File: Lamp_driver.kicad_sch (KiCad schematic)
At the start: 118 parts, among them J302 T44007, J303 T44007, J304 10146581-060_M, J305 T44007, J306 T44007, Q100 MDT7N65, Q301 MPF3N150, Q303 IXYH55N120, Q304 IXYH55N120, Q305 IXYH55N120, U301 IRS2184

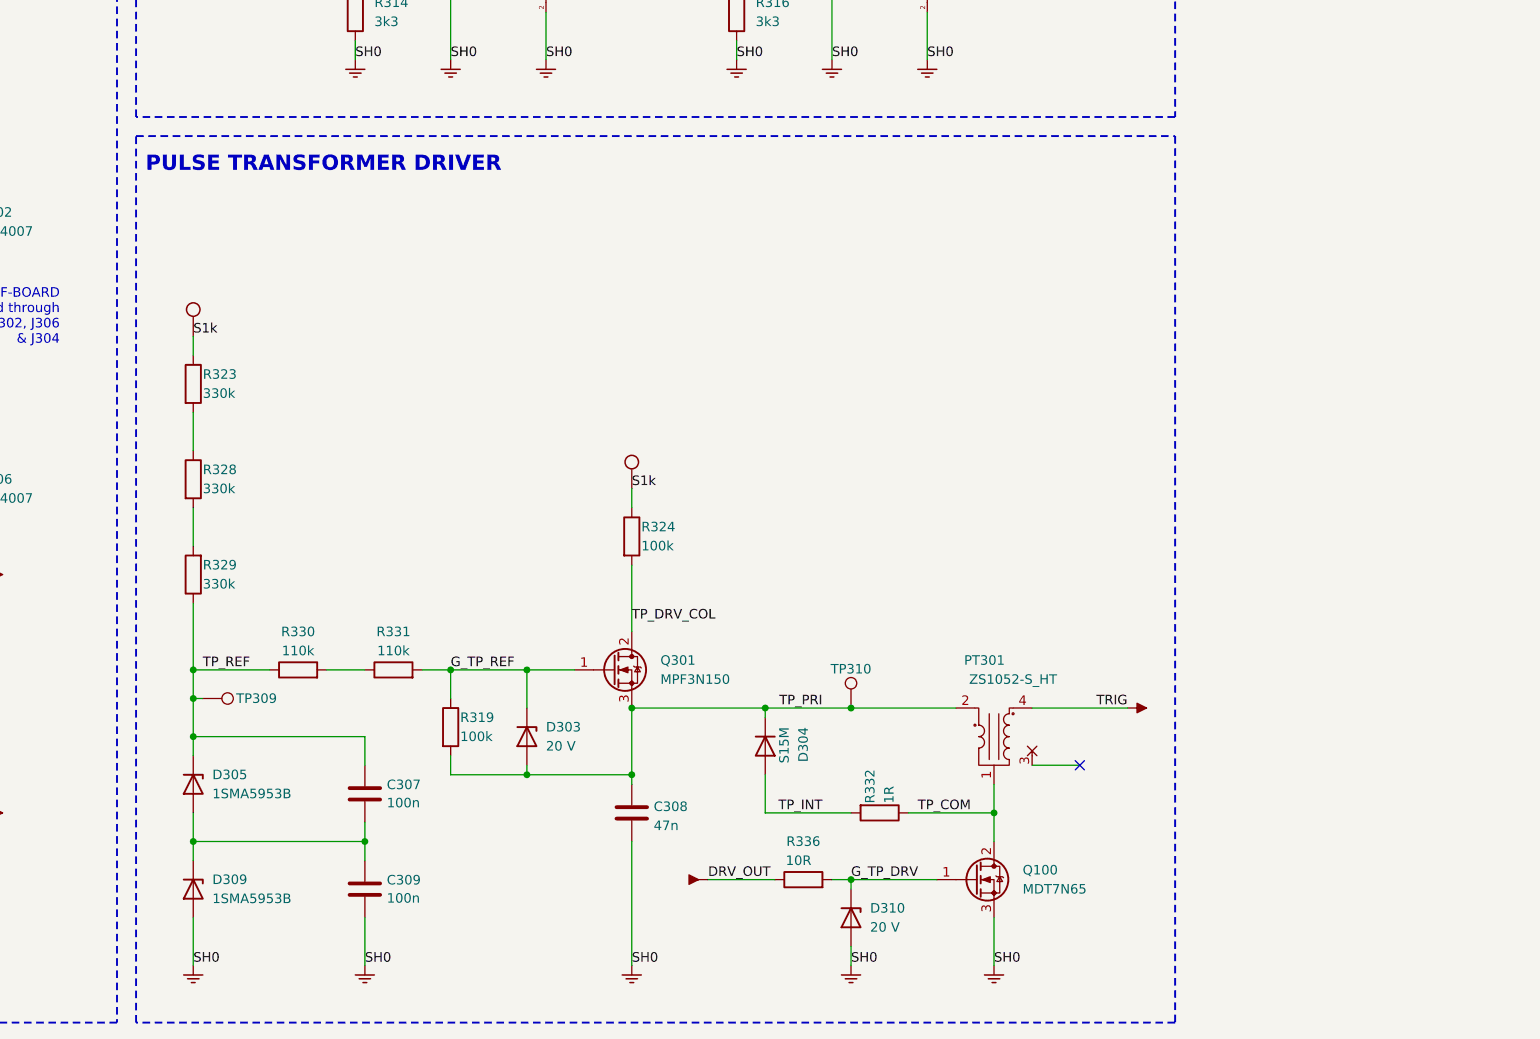
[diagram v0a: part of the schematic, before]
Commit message: Placement updates
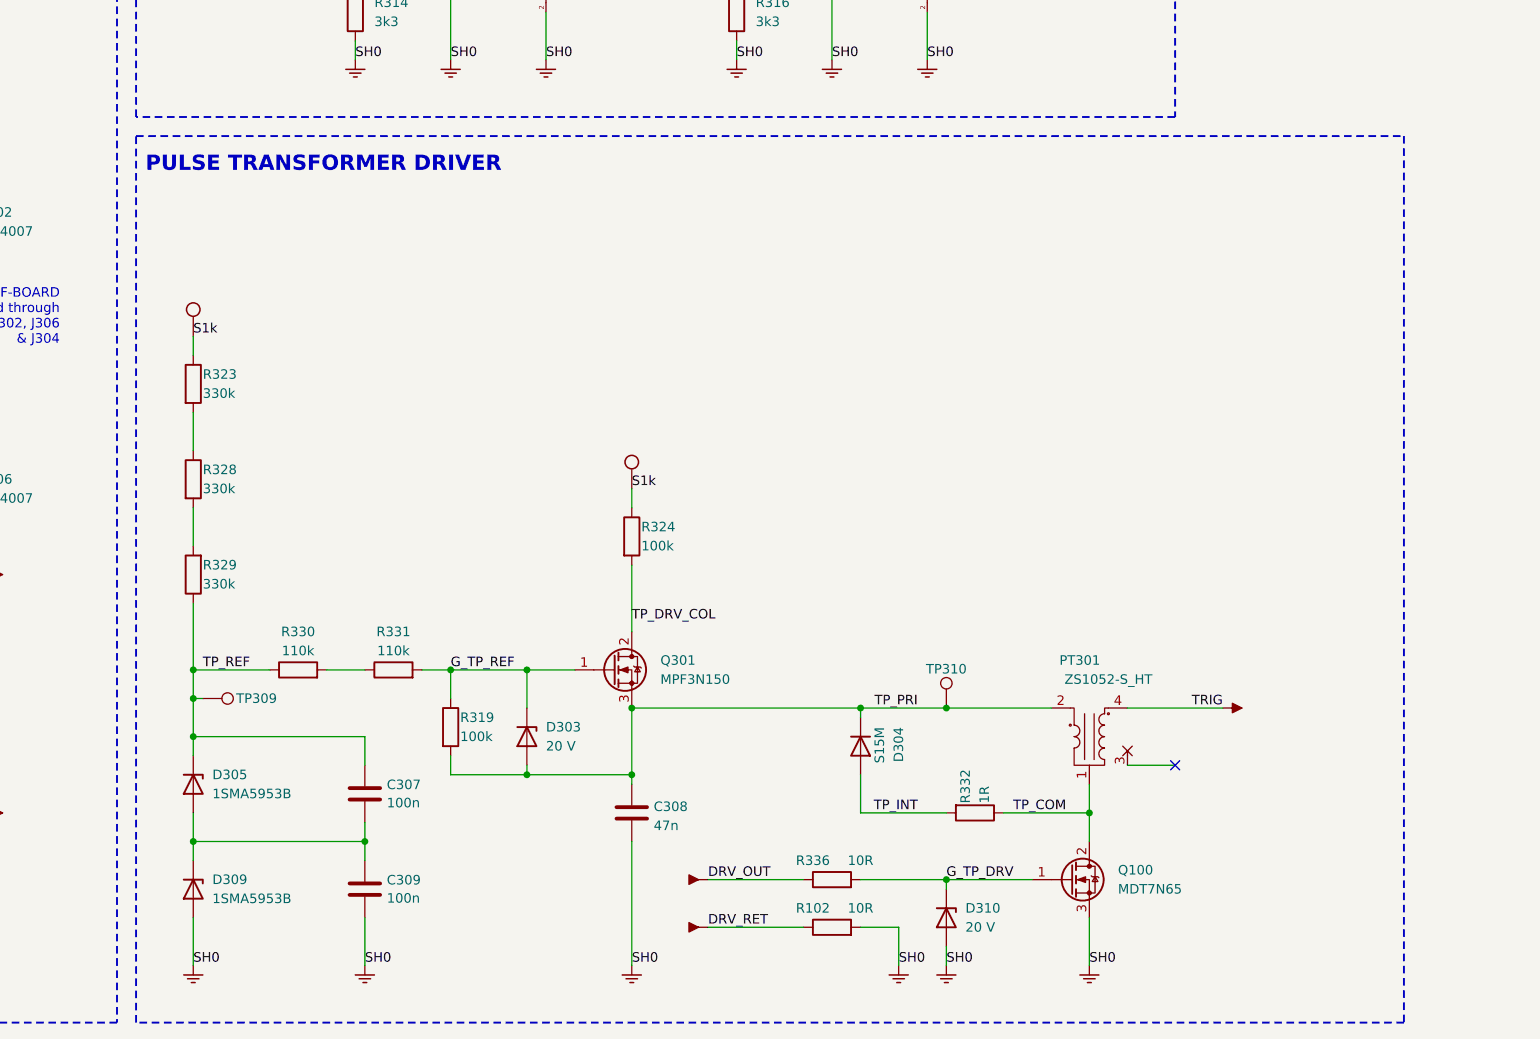
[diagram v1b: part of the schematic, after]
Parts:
- added P137: ~, symbol personal:Cosmetic_IN
- added P138: ~, symbol personal:Cosmetic_GND
- added R102: 10R, Resistor_SMD:R_1206_3216Metric_Pad1.30x1.75mm_HandSolder, symbol Device:R
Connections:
- net DRV_RET: now also P137.1, R102.1
- net SH0: now also P138.1, R102.2
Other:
- moved on the sheet: D304, D310, PT301, Q100, R332, R336, TP310
